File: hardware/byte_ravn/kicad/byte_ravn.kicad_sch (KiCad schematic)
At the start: 8 parts, among them J1 Conn_01x16_Socket, J2 Conn_01x08_Socket, J4 Conn_01x05_Socket, J5 Conn_01x03_Socket, J6 Conn_01x03_Socket, J7 Conn_01x04_Socket, J8 Conn_01x04_Socket, J9 Conn_01x05_Socket

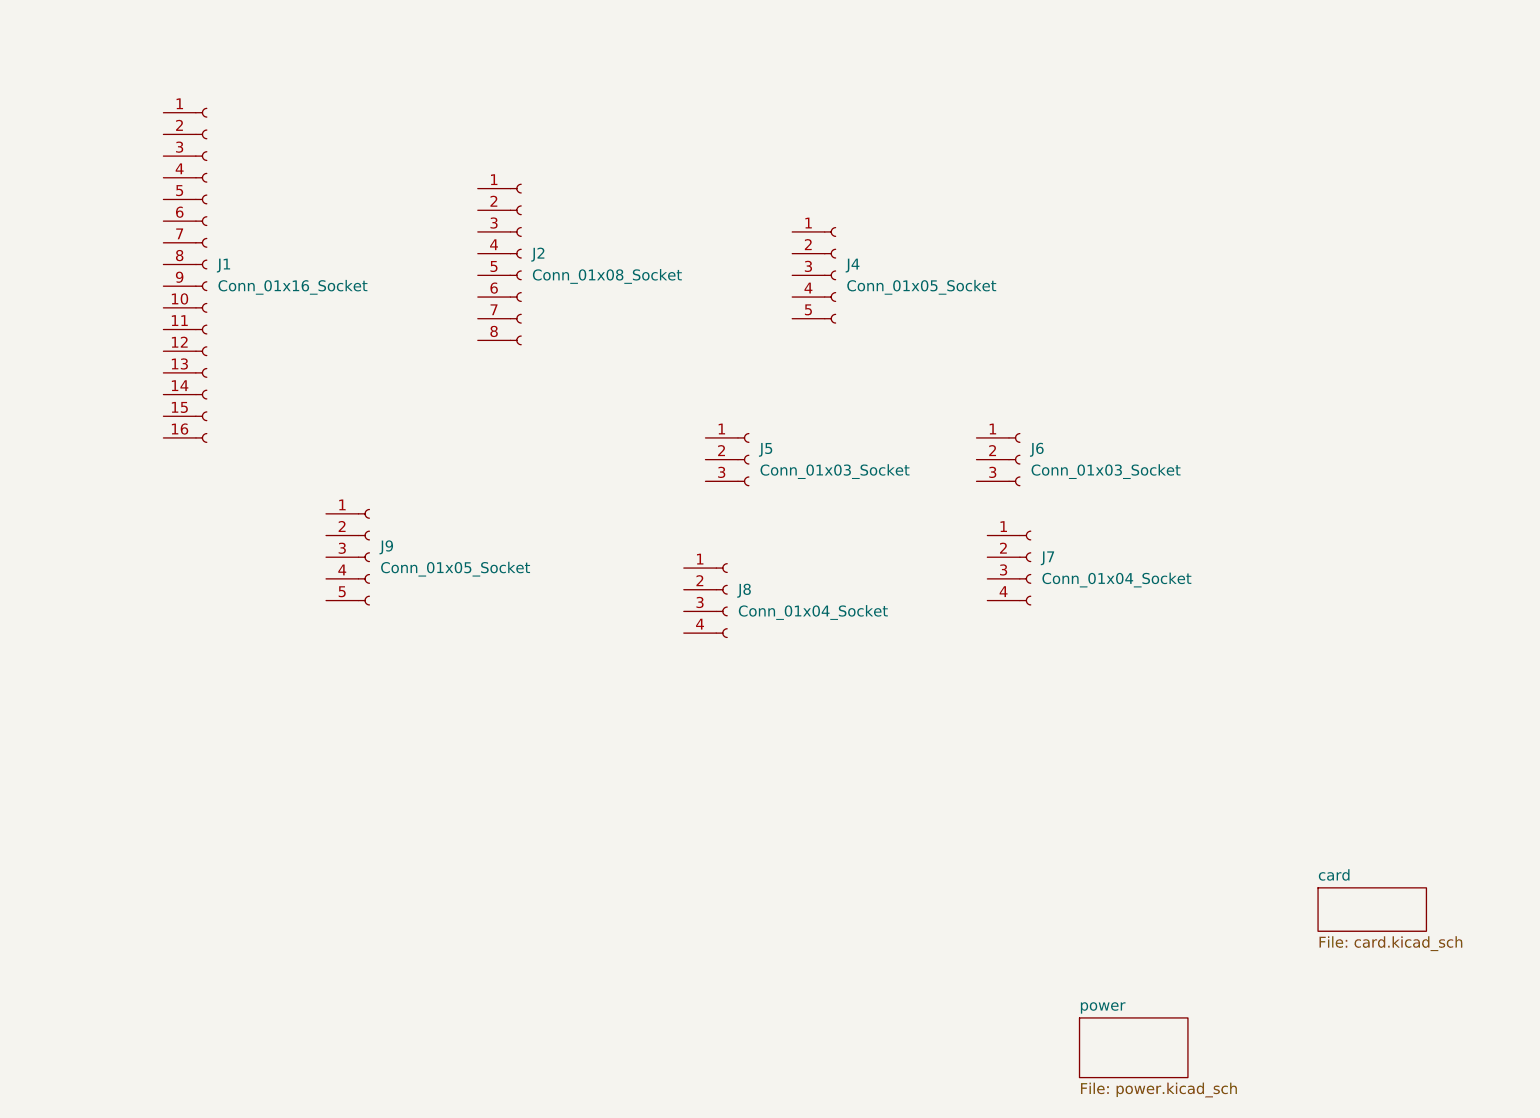
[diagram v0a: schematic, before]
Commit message: Updates to Ravn
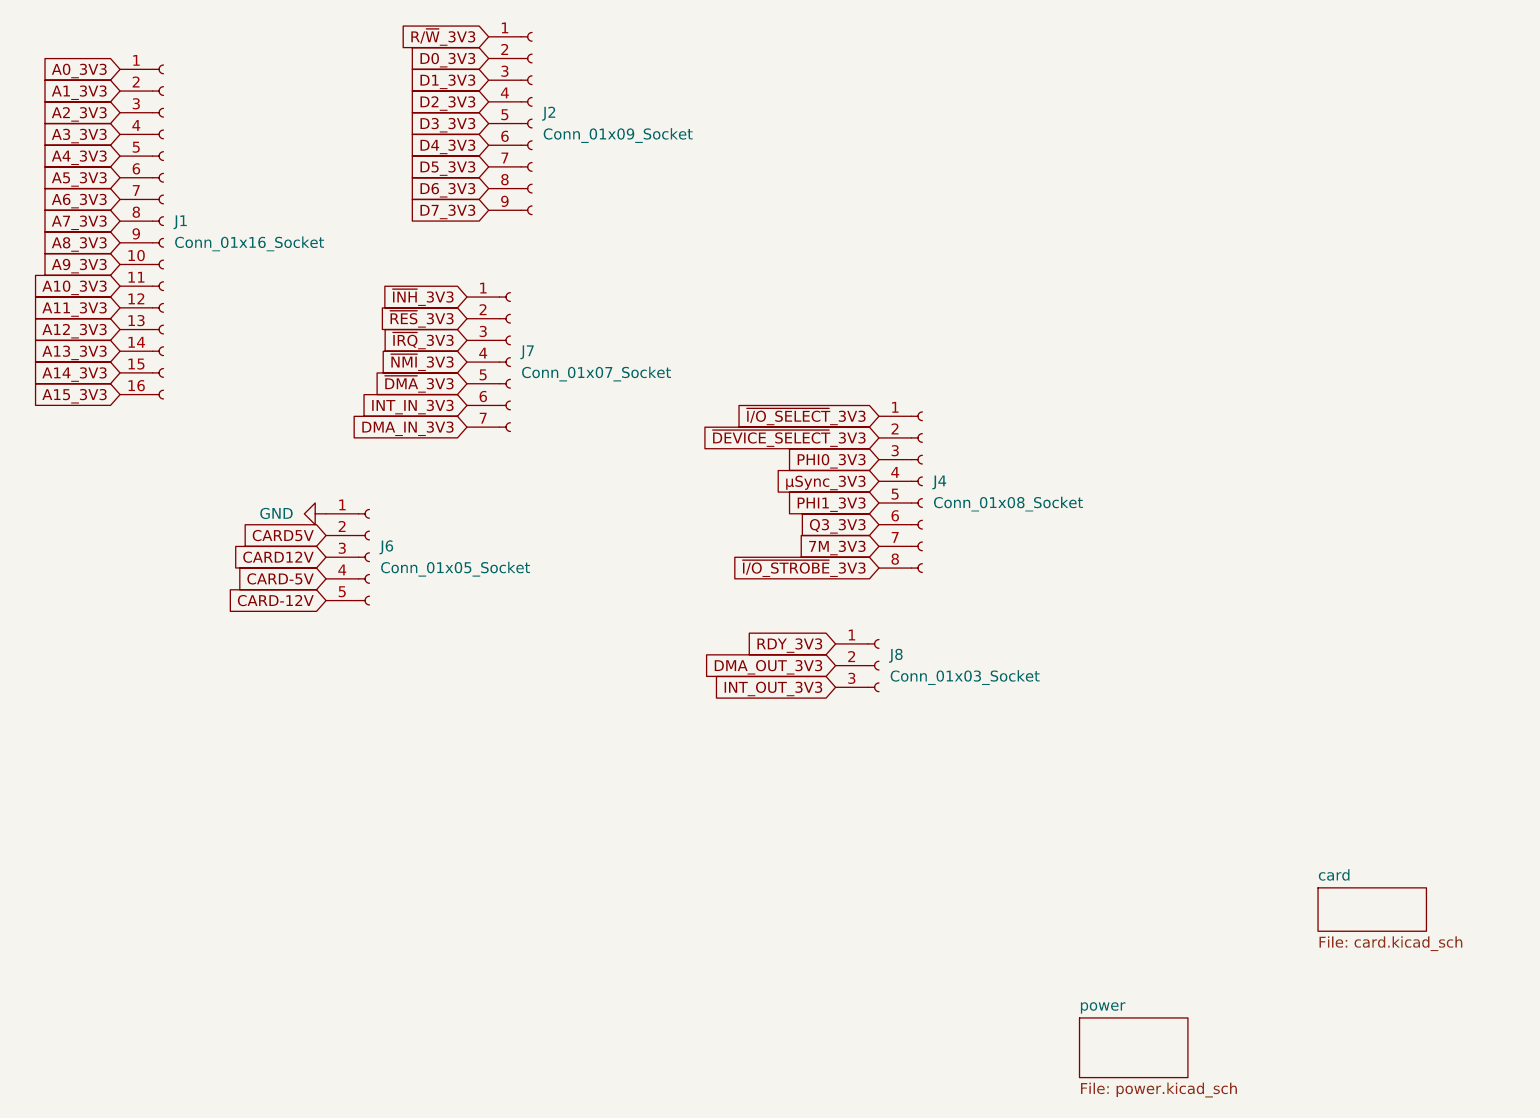
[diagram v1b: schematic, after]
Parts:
- removed J2: Conn_01x08_Socket, Connector_PinHeader_2.54mm:PinHeader_1x08_P2.54mm_Horizontal, symbol Connector:Conn_01x08_Socket
- removed J4: Conn_01x05_Socket, Connector_PinHeader_2.54mm:PinHeader_1x05_P2.54mm_Horizontal, symbol Connector:Conn_01x05_Socket
- removed J5, J6: Conn_01x03_Socket, Connector_PinHeader_2.54mm:PinHeader_1x03_P2.54mm_Horizontal, symbol Connector:Conn_01x03_Socket
- removed J7, J8: Conn_01x04_Socket, Connector_PinHeader_2.54mm:PinHeader_1x04_P2.54mm_Horizontal, symbol Connector:Conn_01x04_Socket
- added J2: Conn_01x09_Socket, Connector_PinHeader_2.54mm:PinHeader_1x09_P2.54mm_Horizontal, symbol Connector:Conn_01x09_Socket
- added J4: Conn_01x08_Socket, Connector_PinHeader_2.54mm:PinHeader_1x08_P2.54mm_Horizontal, symbol Connector:Conn_01x08_Socket
- added J7: Conn_01x07_Socket, Connector_PinHeader_2.54mm:PinHeader_1x07_P2.54mm_Horizontal, symbol Connector:Conn_01x07_Socket
- added J8: Conn_01x03_Socket, Connector_PinHeader_2.54mm:PinHeader_1x03_P2.54mm_Horizontal, symbol Connector:Conn_01x03_Socket
- renumbered J9 to J6
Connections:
- net A0_3V3: now reaches J1.1 (Pin_1)
- net A9_3V3: now reaches J1.10 (Pin_10)
- net A10_3V3: now reaches J1.11 (Pin_11)
- net A11_3V3: now reaches J1.12 (Pin_12)
- net A12_3V3: now reaches J1.13 (Pin_13)
- net A13_3V3: now reaches J1.14 (Pin_14)
- net A14_3V3: now reaches J1.15 (Pin_15)
- net A15_3V3: now reaches J1.16 (Pin_16)
- net A1_3V3: now reaches J1.2 (Pin_2)
- net A2_3V3: now reaches J1.3 (Pin_3)
- net A3_3V3: now reaches J1.4 (Pin_4)
- net A4_3V3: now reaches J1.5 (Pin_5)
- net A5_3V3: now reaches J1.6 (Pin_6)
- net A6_3V3: now reaches J1.7 (Pin_7)
- net A7_3V3: now reaches J1.8 (Pin_8)
- net A8_3V3: now reaches J1.9 (Pin_9)
- net GND: now reaches J6.1 (Pin_1)
- net CARD5V: now reaches J6.2 (Pin_2)
- net CARD12V: now reaches J6.3 (Pin_3)
- net CARD-5V: now reaches J6.4 (Pin_4)
- net CARD-12V: now reaches J6.5 (Pin_5)
- new net 7M_3V3: J4.7 (Pin_7)
- new net D0_3V3: J2.2 (Pin_2)
- new net D1_3V3: J2.3 (Pin_3)
- new net D2_3V3: J2.4 (Pin_4)
- new net D3_3V3: J2.5 (Pin_5)
- new net D4_3V3: J2.6 (Pin_6)
- new net D5_3V3: J2.7 (Pin_7)
- new net D6_3V3: J2.8 (Pin_8)
- new net D7_3V3: J2.9 (Pin_9)
- new net DMA_IN_3V3: J7.7 (Pin_7)
- new net DMA_OUT_3V3: J8.2 (Pin_2)
- new net INT_IN_3V3: J7.6 (Pin_6)
- new net INT_OUT_3V3: J8.3 (Pin_3)
- new net PHI0_3V3: J4.3 (Pin_3)
- new net PHI1_3V3: J4.5 (Pin_5)
- new net Q3_3V3: J4.6 (Pin_6)
- new net RDY_3V3: J8.1 (Pin_1)
- new net R/~{W}_3V3: J2.1 (Pin_1)
- new net ~{DEVICE_SELECT}_3V3: J4.2 (Pin_2)
- new net ~{DMA}_3V3: J7.5 (Pin_5)
- new net ~{INH}_3V3: J7.1 (Pin_1)
- new net ~{IRQ}_3V3: J7.3 (Pin_3)
- new net ~{I/O_SELECT}_3V3: J4.1 (Pin_1)
- new net ~{I/O_STROBE}_3V3: J4.8 (Pin_8)
- new net ~{NMI}_3V3: J7.4 (Pin_4)
- new net ~{RES}_3V3: J7.2 (Pin_2)
- new net µSync_3V3: J4.4 (Pin_4)
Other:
- moved on the sheet: J1
